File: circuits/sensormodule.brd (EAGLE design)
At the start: 27.9 x 58.1 mm, 9 parts, among them U1 ATMEGA328P_PDIP, Y1 16MHz

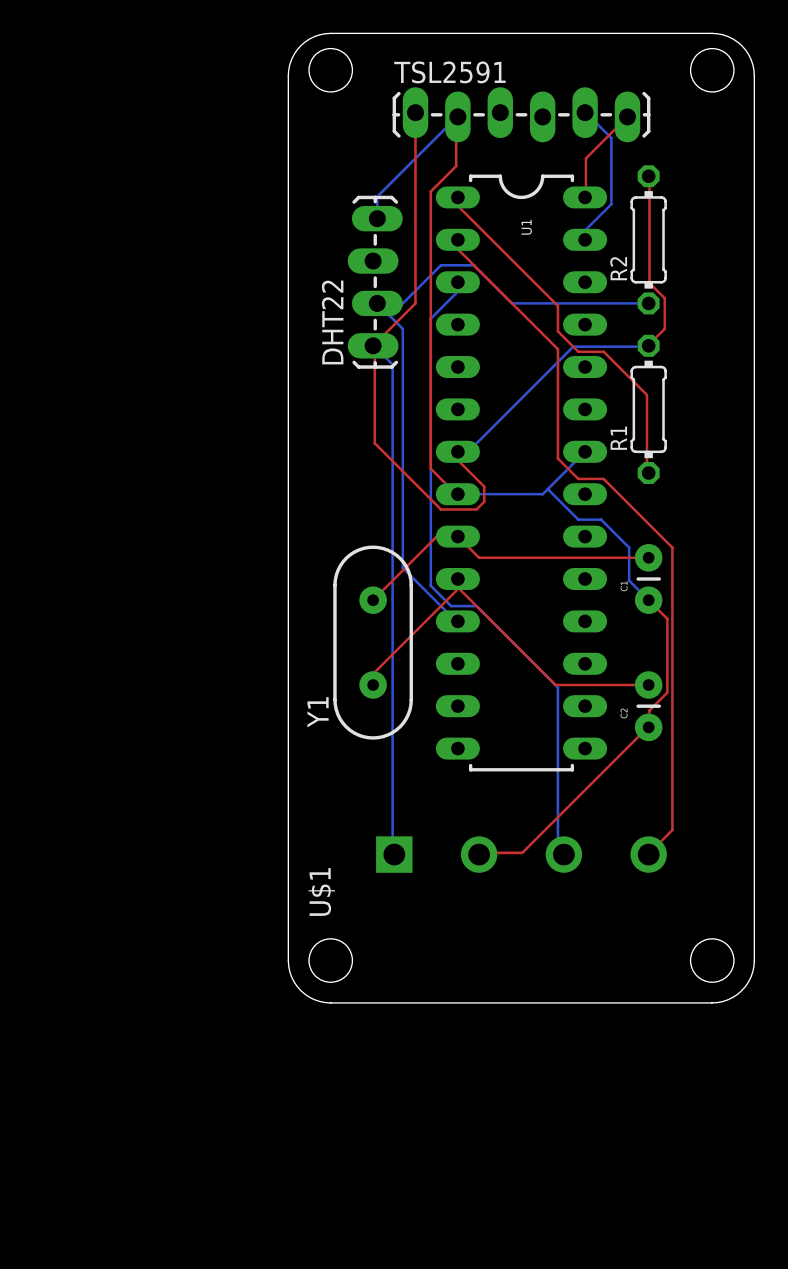
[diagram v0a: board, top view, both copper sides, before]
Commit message: circuit update
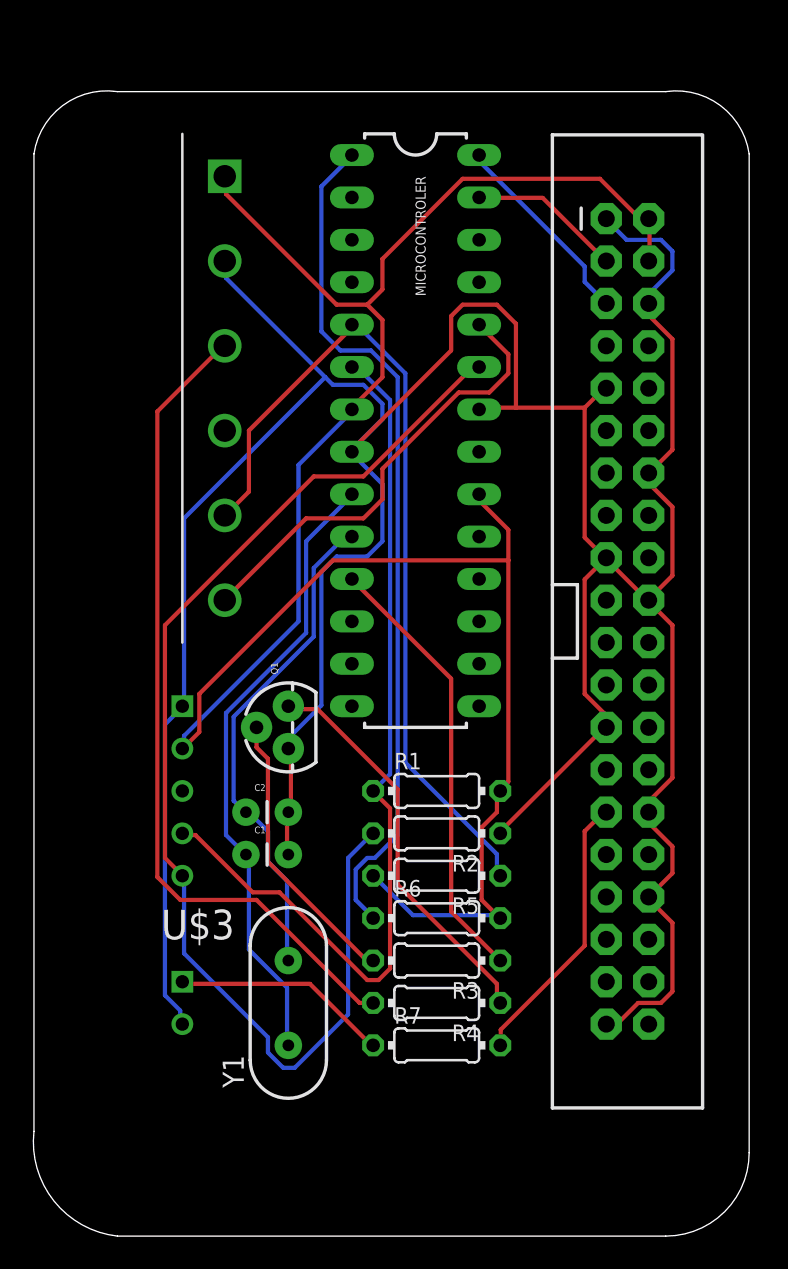
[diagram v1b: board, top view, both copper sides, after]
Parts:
- removed DHT22: (no value), 001_SparkFun-Connectors:1X04_LOCK_LONGPADS
- removed TSL2591: (no value), 001_SparkFun-Connectors:1X06_LOCK_LONGPADS
- removed U$1: UART, 000_CropQuant:I2C_TERM
- removed U1: ATMEGA328P_PDIP, 001_SparkFun-DigitalIC:DIL28-3
- added ENVIRONMENTAL_SENSOR: ENV_OUT, 000_CropQuant:ENV_OUT
- added MICROCONTROLER: ATMEGA328P_PDIP, SparkFun-DigitalIC:DIL28-3
- added Q1: (no value), SparkFun-DiscreteSemi:TO-92
- added R3: 1K, resistor:0204/7
- added R4: 100, resistor:0204/7
- added R5, R6: 4.7K, resistor:0204/7
- added R7: 68, resistor:0204/7
- added SINGLE_BOARD_COMPUTER: RASPBERRYPI-40-PIN-GPIO, 001_SparkFun-Boards:2X20-SHROUDED
- added SOIL_SENSOR: SOIL_OUT, 000_CropQuant:SOIL_OUT
- added U$3: LED, 000_CropQuant:LED
- C1, C2: value 20pF -> 22pF; device 001_SparkFun-Capacitors:CAP-PTH-SMALL -> SparkFun-Capacitors:CAP-PTH-SMALL
- R1: value 4.7k -> 10K
- R2: value 10k -> 10K
- Y1: device 001_SparkFun-FreqCtrl:HC49US -> SparkFun-FreqCtrl:HC49US
- moved R2 37.8 mm to (85.1, 33.0), turned to 180 degrees
- moved C1 28.5 mm to (73.7, 31.8), turned to 0 degrees
- moved R1 26.2 mm to (85.1, 35.6), turned to 0 degrees
- moved C2 24.7 mm to (73.7, 34.3), turned to 0 degrees
- moved Y1 22.2 mm to (76.2, 22.9)
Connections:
- new net 3.3V: C1.2, C2.2, ENVIRONMENTAL_SENSOR.1, MICROCONTROLER.22, MICROCONTROLER.8, Q1.1, R2.1, SINGLE_BOARD_COMPUTER.1, SINGLE_BOARD_COMPUTER.14, SINGLE_BOARD_COMPUTER.17, SINGLE_BOARD_COMPUTER.20, SINGLE_BOARD_COMPUTER.25, SINGLE_BOARD_COMPUTER.30, SINGLE_BOARD_COMPUTER.34, SINGLE_BOARD_COMPUTER.39, SINGLE_BOARD_COMPUTER.6, SINGLE_BOARD_COMPUTER.9, SOIL_SENSOR.2, U$3.2
- new net 5V: ENVIRONMENTAL_SENSOR.2, MICROCONTROLER.20, MICROCONTROLER.7, R1.2, R5.2, R6.2, SINGLE_BOARD_COMPUTER.2, SINGLE_BOARD_COMPUTER.4, SOIL_SENSOR.1
- new net N$11: MICROCONTROLER.24, SOIL_SENSOR.6
- new net N$12: MICROCONTROLER.28, SINGLE_BOARD_COMPUTER.5
- new net N$15: MICROCONTROLER.1, R6.1
- new net N$16: R7.1, U$3.1
- new net N$17: R7.2, SINGLE_BOARD_COMPUTER.29
- net N$1: now also C1.1, MICROCONTROLER.9, Y1.1; no longer R1.1, U1.1
- net N$10: now also R4.2, SOIL_SENSOR.3; no longer U$1.4, U1.2
- net N$2: now also C2.1, MICROCONTROLER.10; no longer C1.2, U1.9
- net N$3: now also Q1.3, R4.1; no longer C2.2, U1.10, Y1.1
- net N$4: now also ENVIRONMENTAL_SENSOR.5, MICROCONTROLER.23; no longer DHT22.1, R1.2, TSL2591.1, U$1.1, U1.7
- net N$5: now also MICROCONTROLER.27, SINGLE_BOARD_COMPUTER.3; no longer DHT22.2, R2.1, U1.11
- net N$6: now also MICROCONTROLER.5, R5.1, SOIL_SENSOR.5; no longer C1.1, C2.1, DHT22.4, TSL2591.2, U$1.2, U1.22, U1.8
- net N$7: now also ENVIRONMENTAL_SENSOR.4, MICROCONTROLER.6, R1.1; no longer TSL2591.5, U1.27
- net N$8: now also MICROCONTROLER.11, R3.1; no longer TSL2591.6, U1.28
- net N$9: now also Q1.2, R3.2; no longer U$1.3, U1.3
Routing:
- net 3.3V: track 0.00 -> 210.6 mm
- net 5V: track 0.00 -> 130.3 mm
- net N$15: track 0.00 -> 51.2 mm
- net N$7: track 8.98 -> 54.5 mm
- net N$5: track 38.9 -> 9.18 mm
- net N$11: track 0.00 -> 27.3 mm
- net N$9: track 39.2 -> 17.1 mm
- net N$6: track 72.8 -> 51.6 mm
- net N$8: track 5.88 -> 26.5 mm
- net N$4: track 89.1 -> 71.4 mm
- net N$17: track 0.00 -> 16.7 mm
- net N$1: track 22.1 -> 37.7 mm
- net N$16: track 0.00 -> 13.0 mm
- net N$12: track 0.00 -> 12.1 mm
- net N$2: track 18.6 -> 30.1 mm
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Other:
- board size 27.9 x 58.1 mm -> 42.9 x 68.6 mm
- board text added: "100"
- board text added: "16MHz"
- board text added: "1k"
- board text added: "68"
- board text added: "ATMEGA328P"
- board text added: "CropQuant"
- board text added: "Sensor Module"
- board text removed: "20pF"
- board text removed: "LIGHT"
- board text removed: "TEMP"
